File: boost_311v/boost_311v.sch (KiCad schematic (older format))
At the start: 42 parts, among them Q1 BC556, Q2 PN2222A, Q3 2N3904, Q4 2N3906, Q5 IRFP260, Q6 2N3904, Q7 2N3906, U1 4N25, U4 LF357, U5 NE555

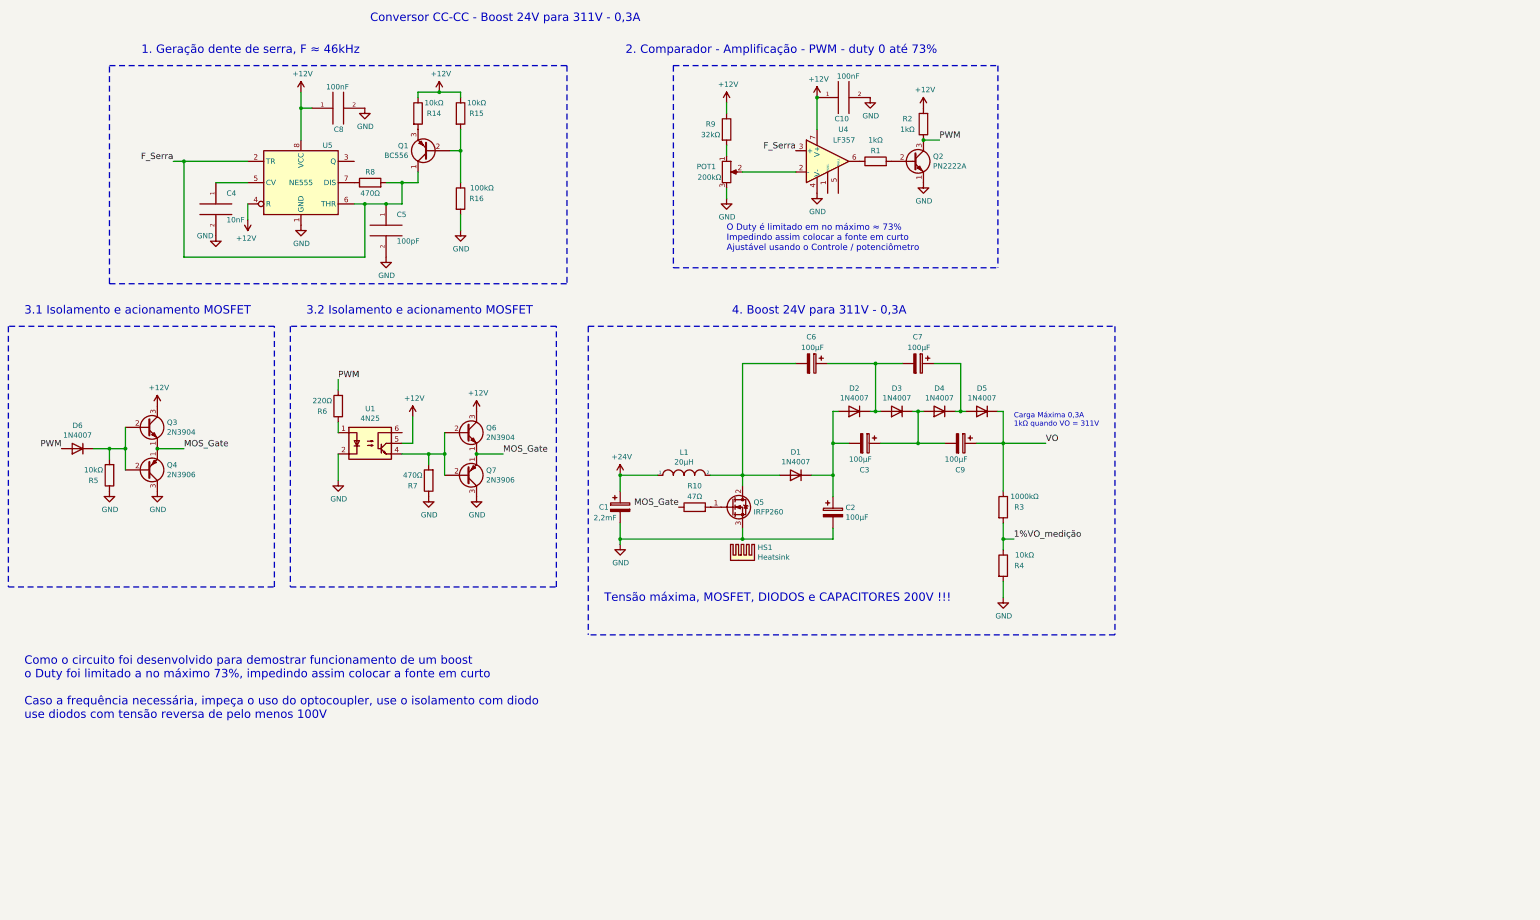
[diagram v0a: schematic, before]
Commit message: Up pcb
Signed-off-by: fgl27 <fglfgl27@gmail.com>
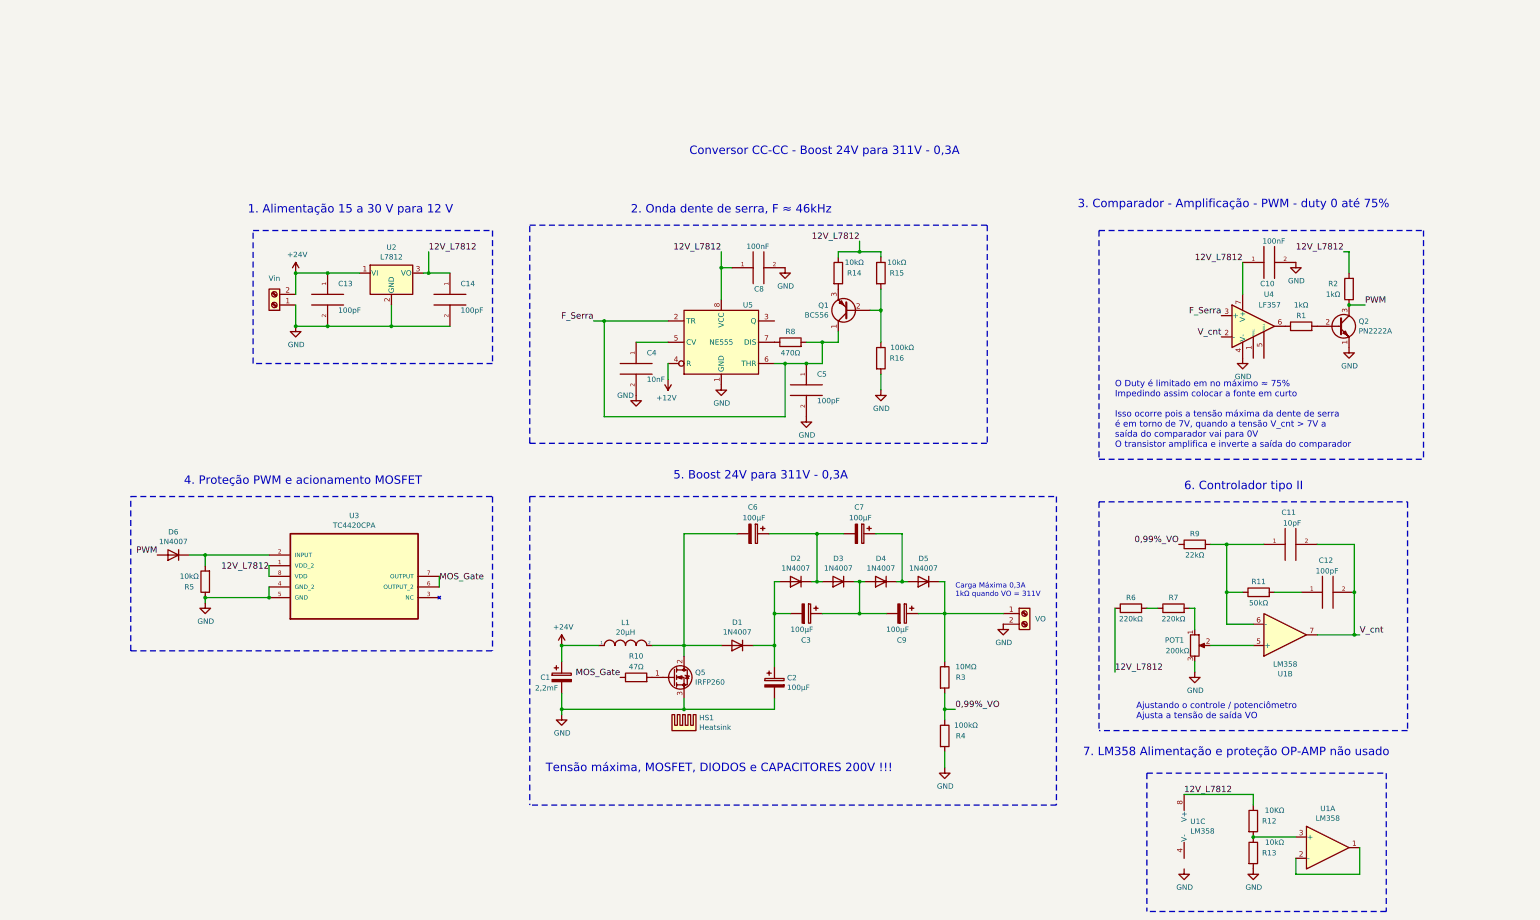
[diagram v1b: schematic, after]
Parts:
- removed Q3, Q6: 2N3904, Package_TO_SOT_THT:TO-92_Inline, symbol Transistor_BJT:2N3904
- removed Q4, Q7: 2N3906, Package_TO_SOT_THT:TO-92_Inline, symbol Transistor_BJT:2N3906
- removed U1: 4N25, Package_DIP:DIP-6_W7.62mm, symbol Isolator:4N25
- added C11: 10pF, Capacitor_THT:C_Disc_D7.5mm_W5.0mm_P5.00mm, symbol pspice:CAP
- added C12, C13, C14: 100pF, Capacitor_THT:C_Disc_D7.5mm_W5.0mm_P5.00mm, symbol pspice:CAP
- added J1: Vin, symbol Connector:Screw_Terminal_01x02
- added J2: VO, symbol Connector:Screw_Terminal_01x02
- added R11: 50kΩ, Resistor_THT:R_Axial_DIN0207_L6.3mm_D2.5mm_P10.16mm_Horizontal, symbol Device:R
- added R12: 10KΩ, Resistor_THT:R_Axial_DIN0207_L6.3mm_D2.5mm_P10.16mm_Horizontal, symbol Device:R
- added R13: 10kΩ, Resistor_THT:R_Axial_DIN0207_L6.3mm_D2.5mm_P10.16mm_Horizontal, symbol Device:R
- added U1: LM358, symbol Amplifier_Operational:LM358
- added U2: L7812, Package_TO_SOT_THT:TO-220-3_Vertical, symbol Regulator_Linear:LM7812_TO220
- added U3: TC4420CPA, DIP254P762X533-8, symbol 4420:TC4420CPA
- R3: value 1000kΩ -> 10MΩ
- R4: value 10kΩ -> 100kΩ
- R6: value 220Ω -> 220kΩ
- R7: value 470Ω -> 220kΩ
- R9: value 32kΩ -> 22kΩ
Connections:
- net +12V: no longer C10.1, C8.1, R14.1, R15.1, R2.2, R9.1, U4.7 (V+), U5.8 (VCC)
- net +24V: now also C13.1, J1.2 (Pin_2), U2.1 (VI)
- net GND: now also C13.2, C14.2, J1.1 (Pin_1), J2.2 (Pin_2), R13.2, U2.2 (GND), U3.4 (GND_2), U3.5 (GND); no longer R7.1
- net MOS_Gate: now also U3.6 (OUTPUT_2), U3.7 (OUTPUT)
- net PWM: no longer R6.2
- net at POT1.1: now also R7.2; no longer R9.2
- net at POT1.2: now also U1.5 (+); no longer U4.2 (-)
- net 12V_L7812: now reaches R6.1
- net 12V_L7812: now also C10.1, C8.1, R14.1, R15.1, R2.2, U4.7 (V+), U5.8 (VCC), C14.1, R12.1, U1.8 (V+), U2.3 (VO), U3.1 (VDD_2), U3.8 (VDD)
- net at D6.1 (K), R5.2: now also U3.2 (INPUT)
- net 1%VO_medição renamed 0,99%_VO
- net 0,99%_VO: now also R9.1
- net VO: no longer names the net of C9.1, D5.1 (K), R3.1
- net VO: now also J2.1 (Pin_1)
- new net: U1.1, U1.2 (-)
- new net: R12.2, R13.1, U1.3 (+)
- new net: C11.1, R11.1, R9.2, U1.6 (-)
- new net: C12.1, R11.2
- new net: R6.2, R7.1
- new net V_cnt: C11.2, C12.2, U1.7, U4.2 (-)
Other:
- note added: "1. Alimentação 15 a 30 V para 12 V"
- note added: "2. Onda dente de serra, F ≈ 46kHz"
- note added: "3. Comparador - Amplificação - PWM - duty 0 até 75%"
- note added: "4. Proteção PWM e acionamento MOSFET"
- note added: "5. Boost 24V para 311V - 0,3A"
- note added: "6. Controlador tipo II"
- note added: "7. LM358 Alimentação e proteção OP-AMP não usado"
- note added: "Ajustando o controle / potenciômetro\nAjusta a tensão de saída VO"
- note added: "O Duty é limitado em no máximo ≈ 75%\nImpedindo assim colocar a fonte em curto\n\nIsso ocorre pois a tensão máxima da dente de serra\né em torno de 7V, quando a tensão V_cnt > 7V a \nsaída do comparador vai para 0V\nO transistor amplifica e inverte a saída do comparador"
- note removed: "1. Geração dente de serra, F ≈ 46kHz"
- note removed: "2. Comparador - Amplificação - PWM - duty 0 até 73%"
- note removed: "3.1 Isolamento e acionamento MOSFET"
- note removed: "3.2 Isolamento e acionamento MOSFET"
- note removed: "4. Boost 24V para 311V - 0,3A"
- note removed: "Como o circuito foi desenvolvido para demostrar funcionamento de um boost\no Duty foi limitado a no máximo 73%, impedindo assim colocar a fonte em curto\n\nCaso a frequência necessária, impeça o uso do optocoupler, use o isolamento com diodo\nuse diodos com tensão reversa de pelo menos 100V"
- note removed: "O Duty é limitado em no máximo ≈ 73%\nImpedindo assim colocar a fonte em curto\nAjustável usando o Controle / potenciômetro"
- moved on the sheet: C1, C10, C2, C3, C4, C5, C6, C7, C8, C9, D1, D2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
